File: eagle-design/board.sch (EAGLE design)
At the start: 13 parts, among them IC1 7805T

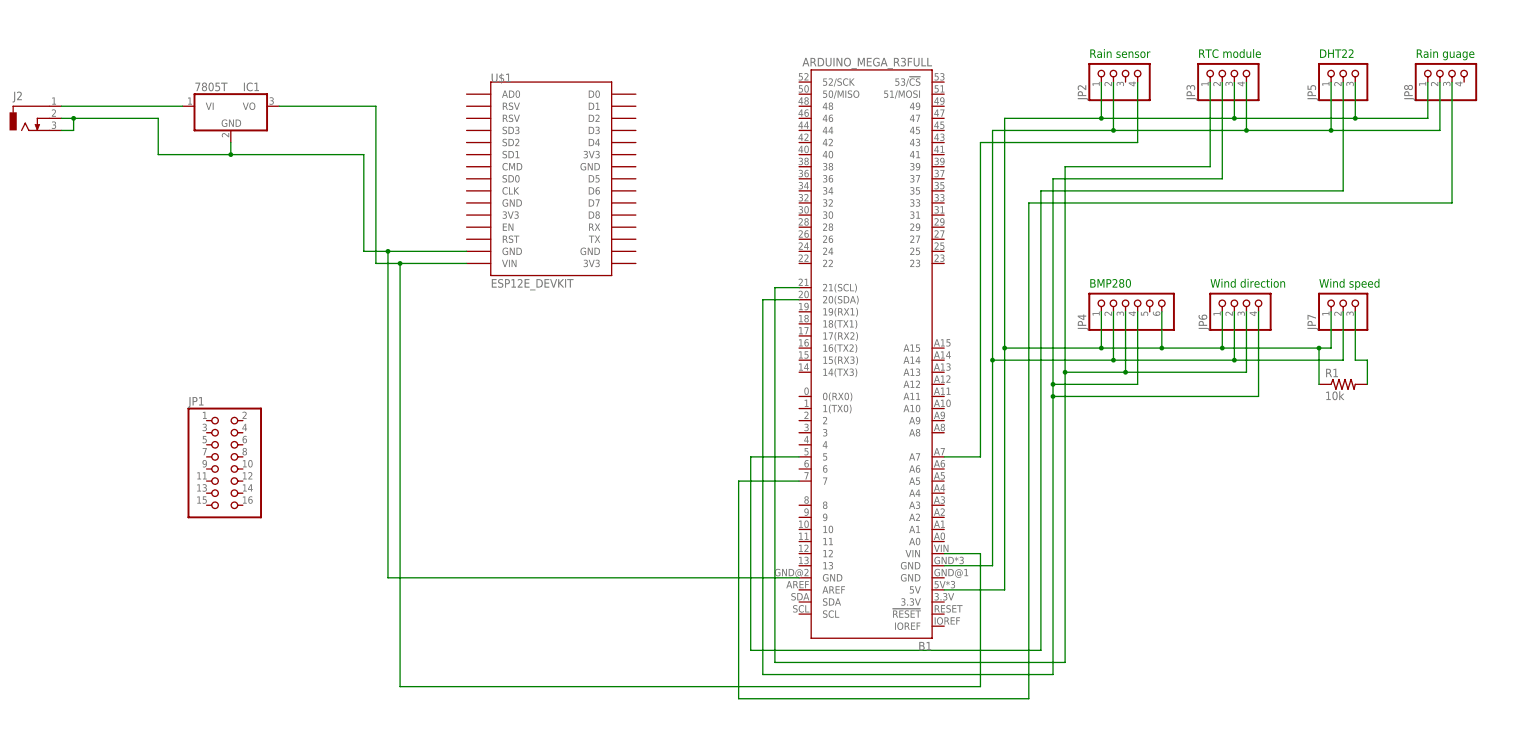
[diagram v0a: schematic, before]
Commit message: Addedd new design
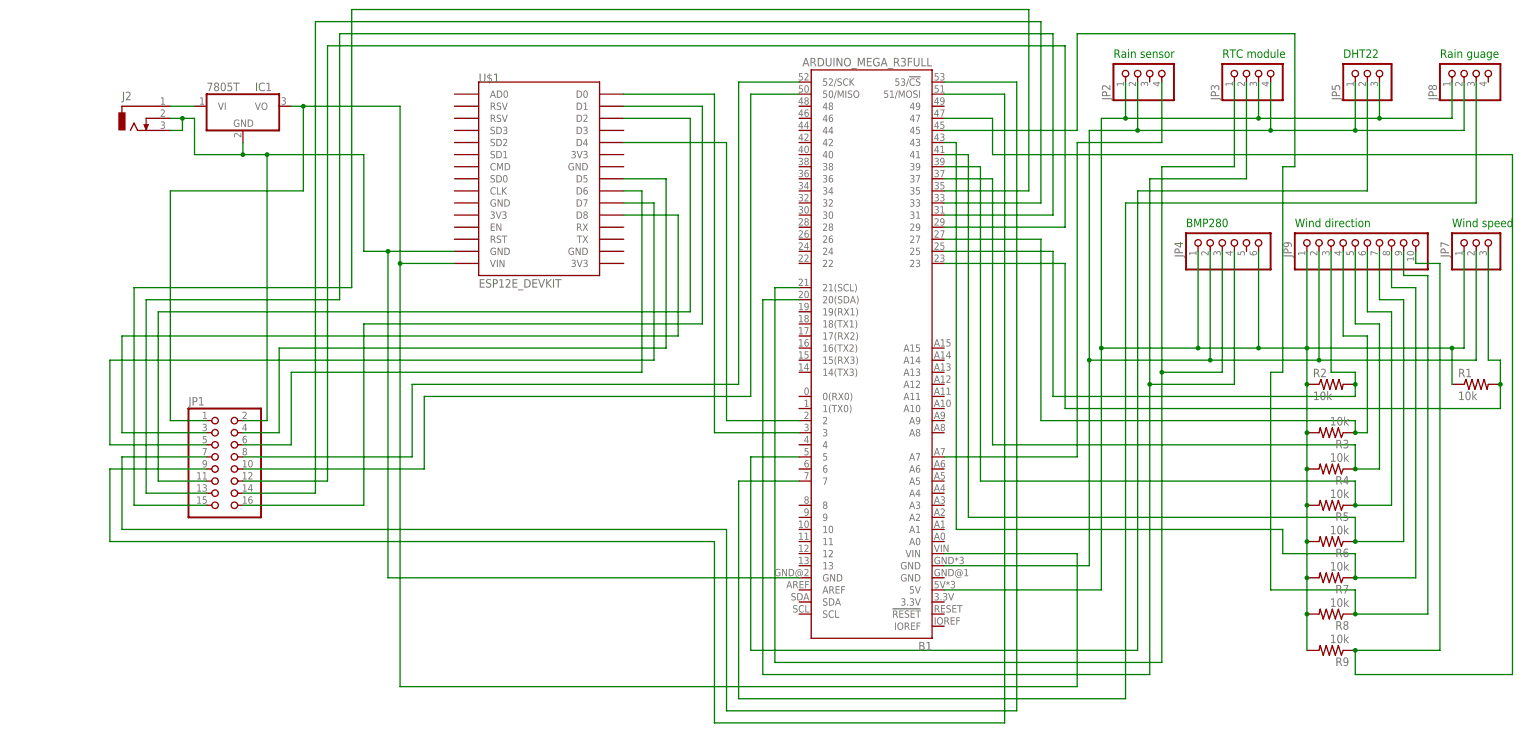
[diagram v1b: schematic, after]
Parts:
- removed JP6: (no value), pinhead:PINHD-1X4
- added JP9: (no value), pinhead:PINHD-1X10
- added R2, R3, R4, R5, R6, R7, R8, R9: 10k, rcl:R-US_0207/10
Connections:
- new net N$13: B1.33, JP1.14
- new net N$14: B1.3, U$1.D0
- new net N$15: JP1.11, U$1.D2
- new net N$16: B1.29, JP1.12
- new net N$17: B1.31, JP1.13
- new net N$18: B1.35, JP1.15
- new net N$19: JP1.16, U$1.D1
- new net N$20: JP1.6, U$1.D6
- new net N$21: JP1.3, U$1.D8
- new net N$22: JP1.4, U$1.D5
- new net N$23: B1.53/!CS, JP1.7
- new net N$24: JP1.5, U$1.D7
- new net N$25: B1.52/SCK, JP1.8
- new net N$26: B1.51/MOSI, JP1.9
- new net N$27: B1.25, JP9.3, R2.2
- new net N$28: B1.50/MISO, JP1.10
- new net N$29: B1.27, JP9.4, R3.1
- new net N$30: B1.37, JP9.5, R4.1
- new net N$31: B1.39, JP9.6, R5.1
- new net N$32: B1.41, JP9.7, R6.1
- new net N$33: B1.43, JP9.8, R7.1
- new net N$34: B1.45, JP9.9, R8.1
- new net N$35: B1.47, JP9.10, R9.1
- new net N$9: B1.2, U$1.D4
- net N$11: no longer JP6.4
- net N$2: now also JP1.2
- net N$3: now also JP9.1, R2.1, R3.2, R4.2, R5.2, R6.2, R7.2, R8.2, R9.2; no longer JP6.1
- net N$4: now also JP1.1
- net N$5: now also B1.23
- net N$6: no longer JP6.3
- net N$7: now also JP9.2; no longer JP6.2
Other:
- moved on the sheet: IC1, J2, JP2, JP3, JP4, JP5, JP7, JP8, R1, U$1
